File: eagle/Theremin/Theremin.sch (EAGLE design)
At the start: 67 parts, among them Q1 2N3904, Q2 2N3904, Q6 2N3904, Q7 2N3904, Q8 2N3904, U1 LM78L12, U2 LM79L12

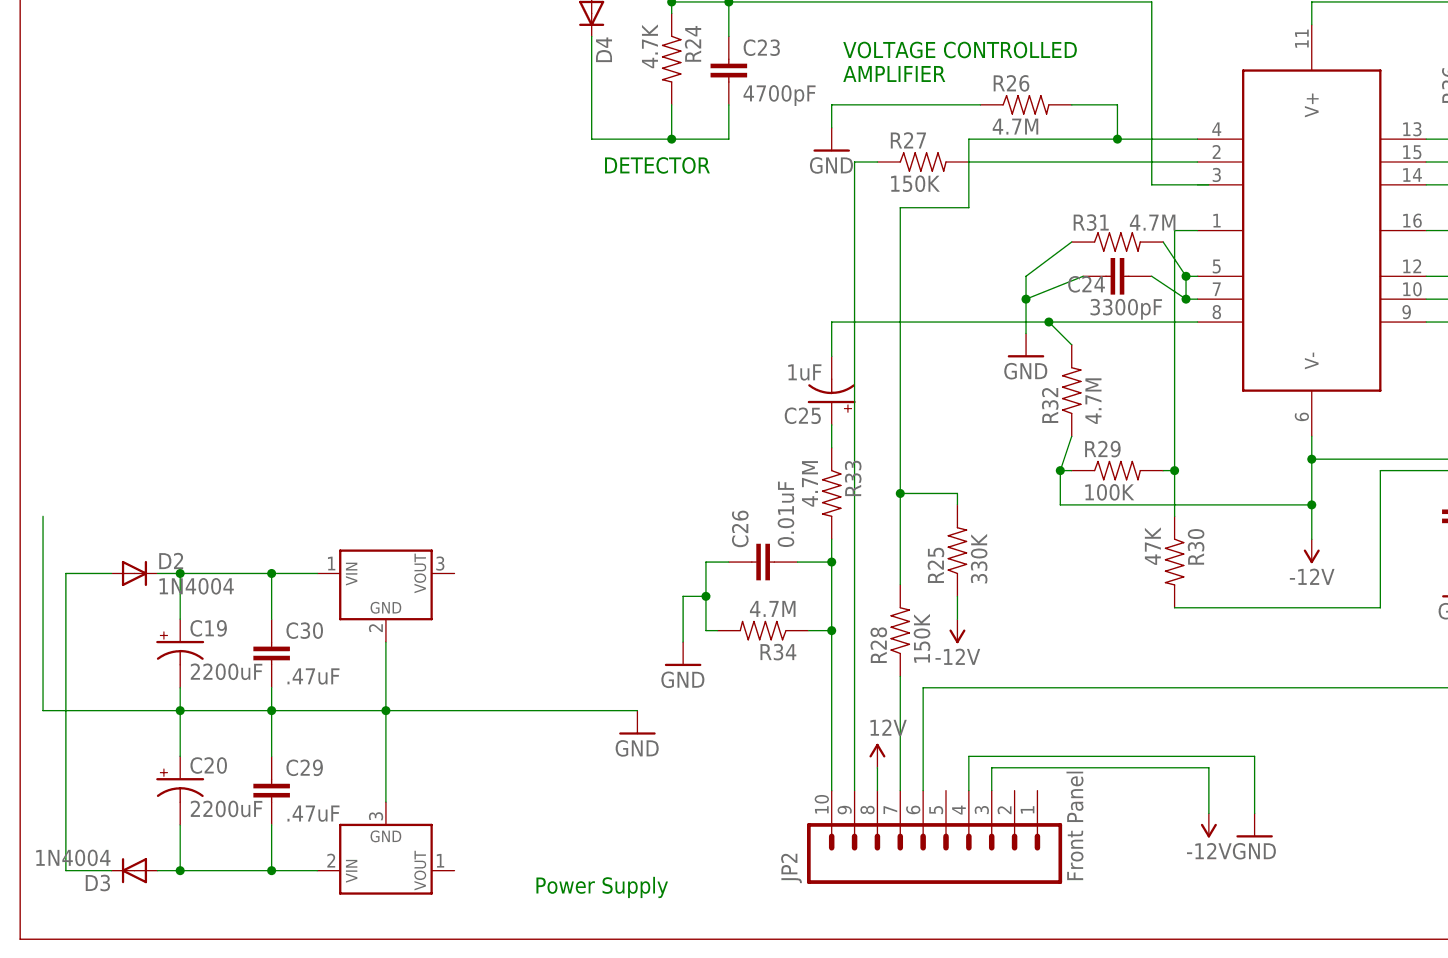
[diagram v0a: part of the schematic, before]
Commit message: work on POWER SUPPLY
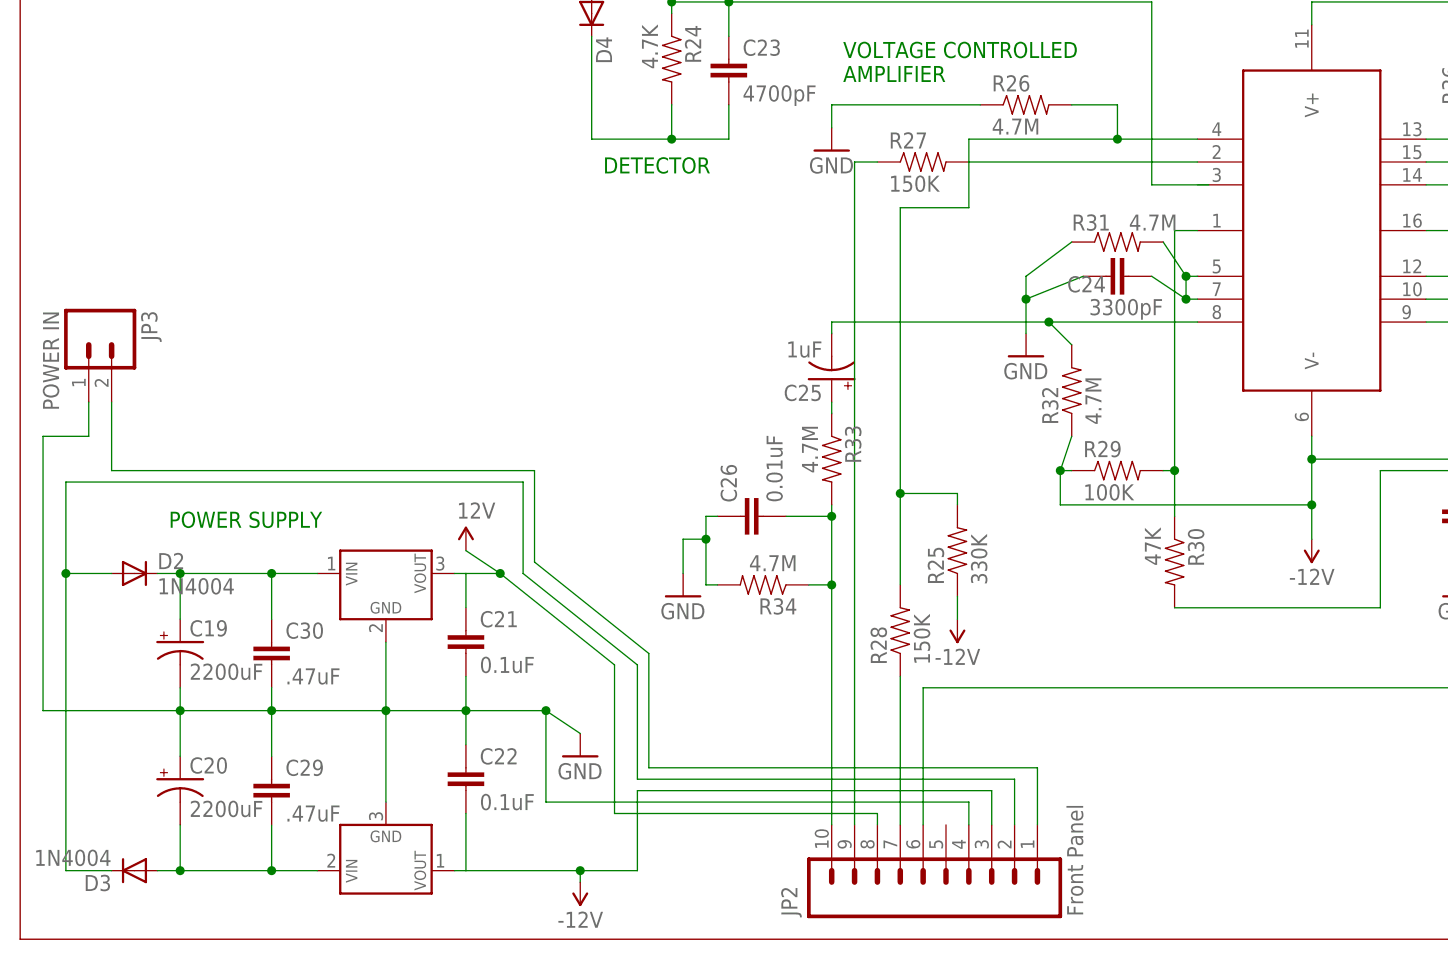
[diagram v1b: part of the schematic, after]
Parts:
- added C21, C22: 0.1uF, SparkFun-Capacitors:CAPPTH
- added JP3: POWER IN, SparkFun-Connectors:M02LOCK
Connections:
- new net N$39: JP2.1, JP3.2
- net -12V: no longer JP2.3
- net 5V: now also C21.1, U1.VOUT
- net GND: now also C21.2, C22.1, JP3.1
- net N$14: now also JP2.2
- net VNEG: now also C22.2, JP2.3, U2.VOUT
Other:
- note added: "POWER SUPPLY"
- note removed: "Power Supply"
- moved on the sheet: C25, C26, JP2, R33, R34
